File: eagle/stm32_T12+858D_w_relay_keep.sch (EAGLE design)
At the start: 100 parts, among them IC1 REG1117, IC2 AD823, IC3 LM328, K1 351, K2 351, T1 BTA41 600B, U1 AT24C32A

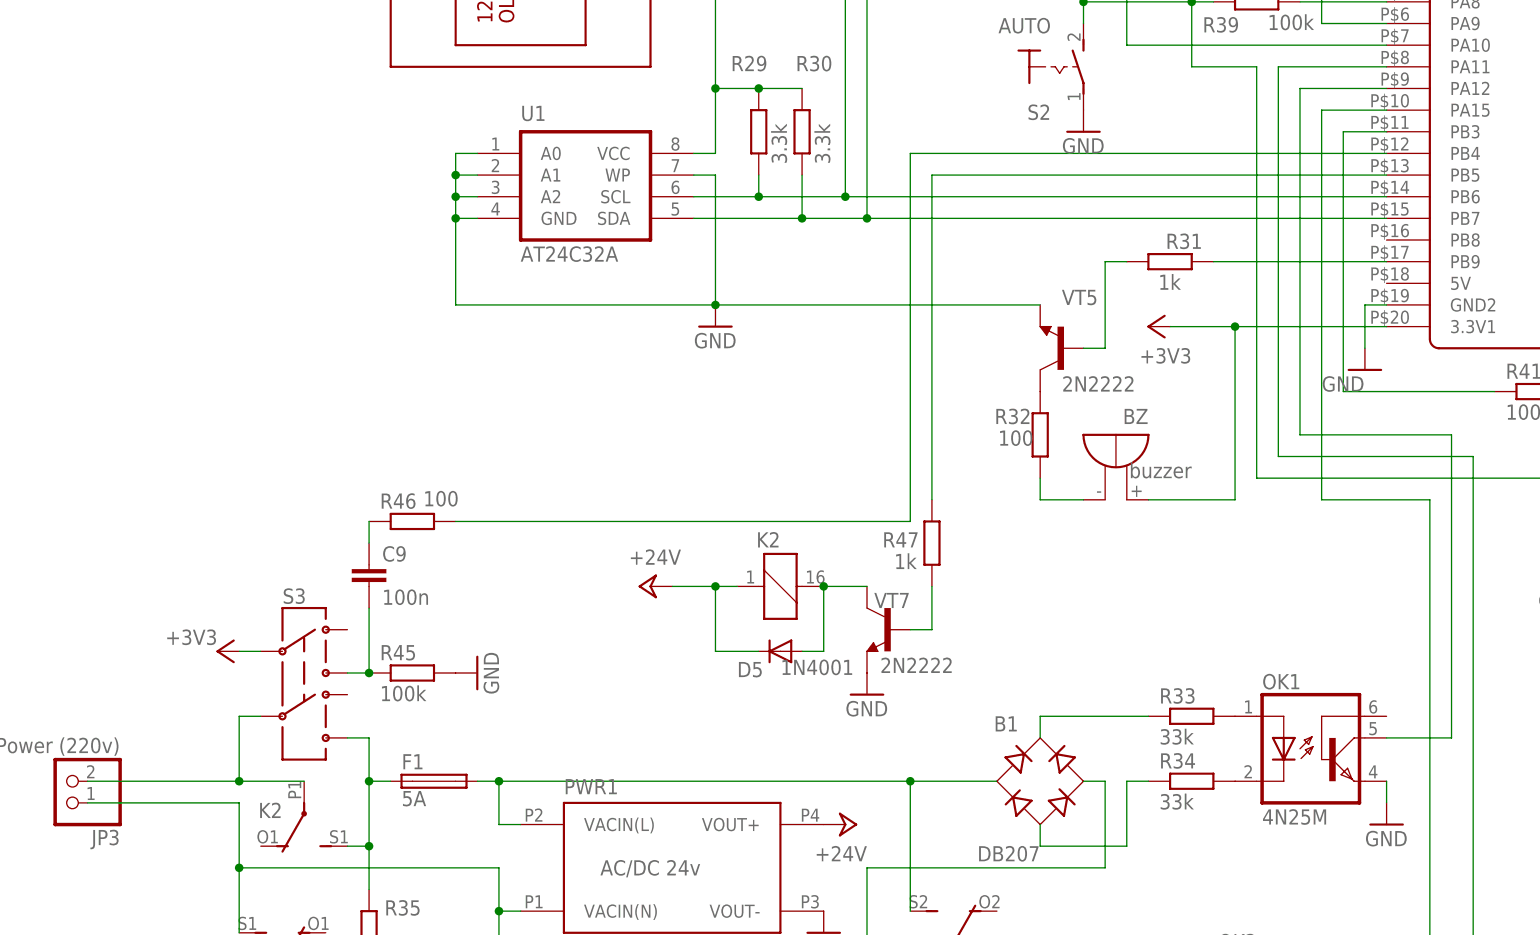
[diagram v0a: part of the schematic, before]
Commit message: Add files via upload
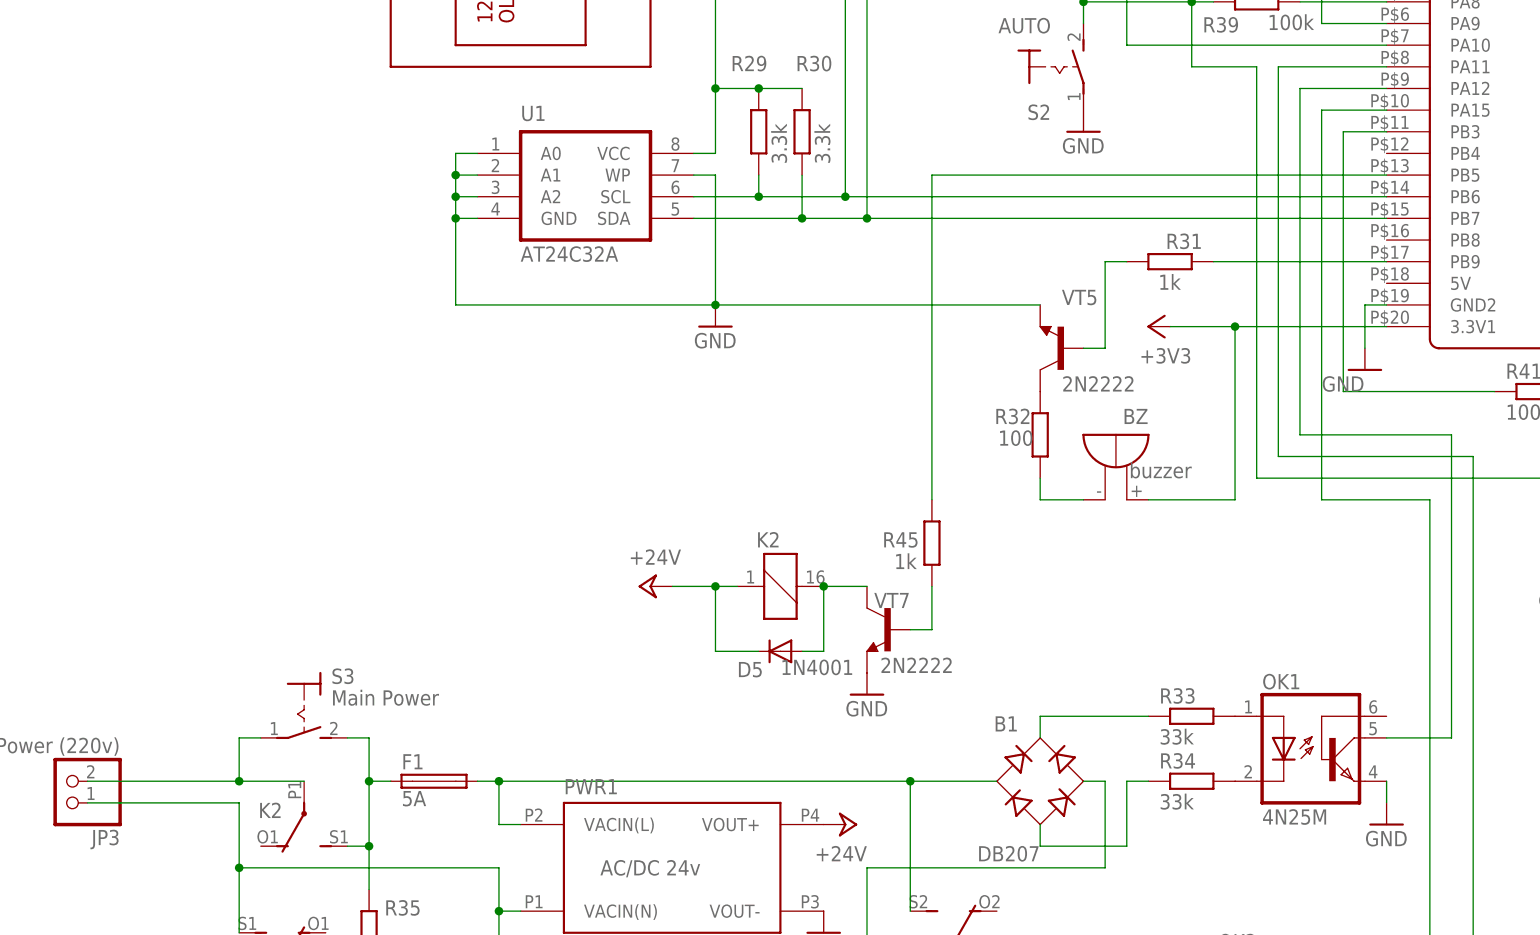
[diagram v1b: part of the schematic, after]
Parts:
- removed C9: 100n, rcl:C-EU025-025X050
- removed R46: 100, rcl:R-EU_0204/5
- removed R47: 1k, rcl:R-EU_0204/5
- R45: value 100k -> 1k
- S3: value (none) -> Main Power; device SparkFun-Retired:SWITCH-DPDTOS -> switch:MS243
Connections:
- removed net N$73: C9.2, R45.1, S3.3
- removed net N$74: C9.1, R46.1
- removed net N$75: R46.2, U$1.PB4
- net +3V3: no longer S3.2
- net GND: no longer R45.2
- net N$62: now also S3.S; no longer S3.6
- net N$70: now also S3.P; no longer S3.5
- net N$76: now also R45.2; no longer R47.2
- net N$77: now also R45.1; no longer R47.1
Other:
- moved on the sheet: R45
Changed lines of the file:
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@@
 <part name="LED1" library="SparkFun" deviceset="LED" device="-3MM-NO_SILK"/>
 <part name="D4" library="diode" library_urn="urn:adsk.eagle:library:210" deviceset="1N4004" device="" package3d_urn="urn:adsk.eagle:package:43336/1" value="1N4001"/>
-<part name="S3" library="SparkFun-Retired" deviceset="SWITCH-DPDT" device="OS"/>
 <part name="K2" library="relay" library_urn="urn:adsk.eagle:library:339" deviceset="351" device="" package3d_urn="urn:adsk.eagle:package:24300/1" value=""/>
-<part name="+3V9" library="supply1" library_urn="urn:adsk.eagle:library:371" deviceset="+3V3" device=""/>
 <part name="PWR1" library="recom-powerline-acdc-converters" deviceset="RAC*SC" device="" technology="02-24" value="AC/DC 24v"/>
 <part name="GND27" library="supply1" library_urn="urn:adsk.eagle:library:371" deviceset="GND" device=""/>
 <part name="P+7" library="supply1" library_urn="urn:adsk.eagle:library:371" deviceset="+24V" device=""/>
-<part name="R45" library="rcl" library_urn="urn:adsk.eagle:library:334" deviceset="R-EU_" device="0204/5" package3d_urn="urn:adsk.eagle:package:23488/1" value="100k"/>
-<part name="GND28" library="supply1" library_urn="urn:adsk.eagle:library:371" deviceset="GND" device=""/>
-<part name="C9" library="rcl" library_urn="urn:adsk.eagle:library:334" deviceset="C-EU" device="025-025X050" package3d_urn="urn:adsk.eagle:package:23629/2" value="100n"/>
-<part name="R46" library="rcl" library_urn="urn:adsk.eagle:library:334" deviceset="R-EU_" device="0204/5" package3d_urn="urn:adsk.eagle:package:23488/1" value="100"/>
-<part name="R47" library="rcl" library_urn="urn:adsk.eagle:library:334" deviceset="R-EU_" device="0204/5" package3d_urn="urn:adsk.eagle:package:23488/1" value="1k"/>
+<part name="R45" library="rcl" library_urn="urn:adsk.eagle:library:334" deviceset="R-EU_" device="0204/5" package3d_urn="urn:adsk.eagle:package:23488/1" value="1k"/>
 <part name="VT7" library="transistor" library_urn="urn:adsk.eagle:library:402" deviceset="2N2222" device="" package3d_urn="urn:adsk.eagle:package:29892/2"/>
 <part name="GND29" library="supply1" library_urn="urn:adsk.eagle:library:371" deviceset="GND" device=""/>
 <part name="D5" library="diode" library_urn="urn:adsk.eagle:library:210" deviceset="1N4004" device="" package3d_urn="urn:adsk.eagle:package:43336/1" value="1N4001"/>
 <part name="P+8" library="supply1" library_urn="urn:adsk.eagle:library:371" deviceset="+24V" device=""/>
+<part name="S3" library="switch" library_urn="urn:adsk.eagle:library:380" deviceset="MS243" device="" package3d_urn="urn:adsk.eagle:package:27683/1" value="Main Power"/>
 </parts>
 <sheets>
@@
 <attribute name="VALUE" x="-78.74" y="-86.1314" size="1.778" layer="96" rot="R180"/>
 </instance>
-<instance part="S3" gate="G$1" x="-109.22" y="-12.7" smashed="yes">
-<attribute name="NAME" x="-111.76" y="-4.572" size="1.778" layer="95"/>
-<attribute name="VALUE" x="-111.76" y="-25.4" size="1.778" layer="96"/>
-</instance>
 <instance part="K2" gate="1" x="-53.34" y="-2.54" smashed="yes" rot="R90">
 <attribute name="VALUE" x="-53.721" y="-8.89" size="1.778" layer="96" rot="R180"/>
@@
 <attribute name="PART" x="-111.76" y="-27.94" size="1.778" layer="95" rot="R180"/>
 </instance>
-<instance part="+3V9" gate="G$1" x="-119.38" y="-10.16" smashed="yes" rot="R90">
-<attribute name="VALUE" x="-119.38" y="-7.62" size="1.778" layer="96" rot="R180"/>
-</instance>
 <instance part="PWR1" gate="_MODULE" x="-66.04" y="-35.56" smashed="yes">
 <attribute name="VALUE" x="-68.58" y="-35.56" size="1.778" layer="96" align="center"/>
@@
 <attribute name="VALUE" x="-43.18" y="-33.02" size="1.778" layer="96" rot="R180"/>
 </instance>
-<instance part="R45" gate="G$1" x="-96.52" y="-12.7" smashed="yes">
-<attribute name="NAME" x="-100.33" y="-11.2014" size="1.778" layer="95"/>
-<attribute name="VALUE" x="-100.33" y="-16.002" size="1.778" layer="96"/>
-</instance>
-<instance part="GND28" gate="1" x="-88.9" y="-12.7" smashed="yes" rot="R90">
-<attribute name="VALUE" x="-86.36" y="-15.24" size="1.778" layer="96" rot="R90"/>
-</instance>
-<instance part="C9" gate="G$1" x="-101.6" y="0" smashed="yes">
-<attribute name="NAME" x="-100.076" y="0.381" size="1.778" layer="95"/>
-<attribute name="VALUE" x="-100.076" y="-4.699" size="1.778" layer="96"/>
-</instance>
-<instance part="R46" gate="G$1" x="-96.52" y="5.08" smashed="yes">
-<attribute name="NAME" x="-100.33" y="6.5786" size="1.778" layer="95"/>
-<attribute name="VALUE" x="-95.25" y="6.858" size="1.778" layer="96"/>
-</instance>
-<instance part="R47" gate="G$1" x="-35.56" y="2.54" smashed="yes" rot="R90">
+<instance part="R45" gate="G$1" x="-35.56" y="2.54" smashed="yes" rot="R90">
 <attribute name="NAME" x="-37.0586" y="3.81" size="1.778" layer="95" rot="R180"/>
 <attribute name="VALUE" x="-37.338" y="1.27" size="1.778" layer="96" rot="R180"/>
@@
 <instance part="P+8" gate="1" x="-68.58" y="-2.54" smashed="yes" rot="R90">
 <attribute name="VALUE" x="-71.12" y="0" size="1.778" layer="96"/>
+</instance>
+<instance part="S3" gate="1" x="-109.22" y="-17.78" smashed="yes" rot="R270">
+<attribute name="NAME" x="-106.045" y="-13.97" size="1.778" layer="95"/>
+<attribute name="VALUE" x="-106.045" y="-16.51" size="1.778" layer="96"/>
 </instance>
 </instances>
@@
 <pinref part="+3V5" gate="G$1" pin="+3V3"/>
 <wire x1="-17.78" y1="81.28" x2="-17.78" y2="83.82" width="0.1524" layer="91"/>
-</segment>
-<segment>
-<pinref part="+3V9" gate="G$1" pin="+3V3"/>
-<pinref part="S3" gate="G$1" pin="2"/>
-<wire x1="-116.84" y1="-10.16" x2="-114.3" y2="-10.16" width="0.1524" layer="91"/>
 </segment>
 </net>
@@
 </segment>
 <segment>
-<pinref part="R45" gate="G$1" pin="2"/>
-<pinref part="GND28" gate="1" pin="GND"/>
-</segment>
-<segment>
 <pinref part="VT7" gate="G$1" pin="E"/>
 <pinref part="GND29" gate="1" pin="GND"/>
@@
 <net name="N$70" class="0">
 <segment>
-<wire x1="-116.84" y1="-25.4" x2="-116.84" y2="-17.78" width="0.1524" layer="91"/>
-<pinref part="S3" gate="G$1" pin="5"/>
-<wire x1="-116.84" y1="-17.78" x2="-114.3" y2="-17.78" width="0.1524" layer="91"/>
 <pinref part="K2" gate="2" pin="P"/>
-<wire x1="-116.84" y1="-25.4" x2="-109.22" y2="-25.4" width="0.1524" layer="91"/>
 <pinref part="JP3" gate="G$1" pin="2"/>
 <wire x1="-134.62" y1="-25.4" x2="-116.84" y2="-25.4" width="0.1524" layer="91"/>
+<pinref part="S3" gate="1" pin="P"/>
+<wire x1="-116.84" y1="-25.4" x2="-109.22" y2="-25.4" width="0.1524" layer="91"/>
+<wire x1="-114.3" y1="-20.32" x2="-116.84" y2="-20.32" width="0.1524" layer="91"/>
+<wire x1="-116.84" y1="-20.32" x2="-116.84" y2="-25.4" width="0.1524" layer="91"/>
 <junction x="-116.84" y="-25.4"/>
 </segment>
@@
 <junction x="-101.6" y="-33.02"/>
 <wire x1="-101.6" y1="-33.02" x2="-101.6" y2="-25.4" width="0.1524" layer="91"/>
-<pinref part="S3" gate="G$1" pin="6"/>
 <wire x1="-101.6" y1="-25.4" x2="-101.6" y2="-20.32" width="0.1524" layer="91"/>
 <wire x1="-104.14" y1="-20.32" x2="-101.6" y2="-20.32" width="0.1524" layer="91"/>
@@
 <wire x1="-99.06" y1="-25.4" x2="-101.6" y2="-25.4" width="0.1524" layer="91"/>
 <junction x="-101.6" y="-25.4"/>
+<pinref part="S3" gate="1" pin="S"/>
 </segment>
 </net>
@@
 </segment>
 </net>
-<net name="N$73" class="0">
-<segment>
-<pinref part="S3" gate="G$1" pin="3"/>
-<pinref part="R45" gate="G$1" pin="1"/>
-<wire x1="-104.14" y1="-12.7" x2="-101.6" y2="-12.7" width="0.1524" layer="91"/>
-<pinref part="C9" gate="G$1" pin="2"/>
-<wire x1="-101.6" y1="-12.7" x2="-101.6" y2="-5.08" width="0.1524" layer="91"/>
-<junction x="-101.6" y="-12.7"/>
-</segment>
-</net>
-<net name="N$74" class="0">
-<segment>
-<pinref part="C9" gate="G$1" pin="1"/>
-<pinref part="R46" gate="G$1" pin="1"/>
-<wire x1="-101.6" y1="2.54" x2="-101.6" y2="5.08" width="0.1524" layer="91"/>
-</segment>
-</net>
-<net name="N$75" class="0">
-<segment>
-<pinref part="R46" gate="G$1" pin="2"/>
-<wire x1="-91.44" y1="5.08" x2="-38.1" y2="5.08" width="0.1524" layer="91"/>
-<wire x1="-38.1" y1="5.08" x2="-38.1" y2="48.26" width="0.1524" layer="91"/>
-<pinref part="U$1" gate="G$1" pin="PB4"/>
-<wire x1="-38.1" y1="48.26" x2="17.78" y2="48.26" width="0.1524" layer="91"/>
-</segment>
-</net>
 <net name="N$76" class="0">
 <segment>
@@
 <wire x1="17.78" y1="45.72" x2="-35.56" y2="45.72" width="0.1524" layer="91"/>
 <wire x1="-35.56" y1="45.72" x2="-35.56" y2="7.62" width="0.1524" layer="91"/>
-<pinref part="R47" gate="G$1" pin="2"/>
+<pinref part="R45" gate="G$1" pin="2"/>
 </segment>
 </net>
@@
 <pinref part="VT7" gate="G$1" pin="B"/>
 <wire x1="-38.1" y1="-7.62" x2="-35.56" y2="-7.62" width="0.1524" layer="91"/>
-<pinref part="R47" gate="G$1" pin="1"/>
+<pinref part="R45" gate="G$1" pin="1"/>
 <wire x1="-35.56" y1="-7.62" x2="-35.56" y2="-2.54" width="0.1524" layer="91"/>
 </segment>
